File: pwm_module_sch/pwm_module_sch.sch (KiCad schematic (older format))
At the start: 47 parts, among them J1 SWIMM, J2 output -, J3 input, J4 output+, Q1 AO3400, Q2 6N60, SW1 ., SW2 ., U1 TM1637, U2 STM8S003F3P, U3 LM358, U4 L78L33

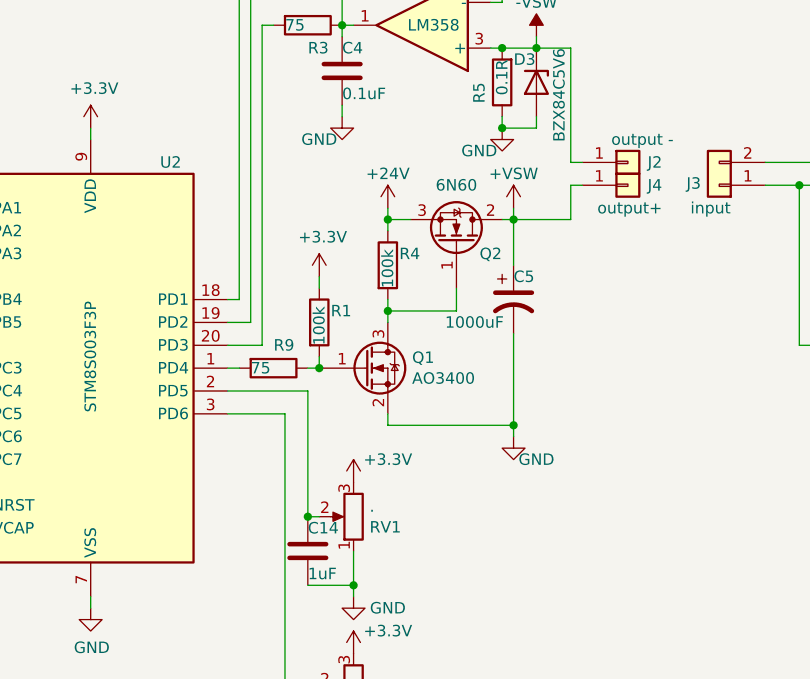
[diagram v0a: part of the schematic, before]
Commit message: low lewel written, not tested, todo: main menu
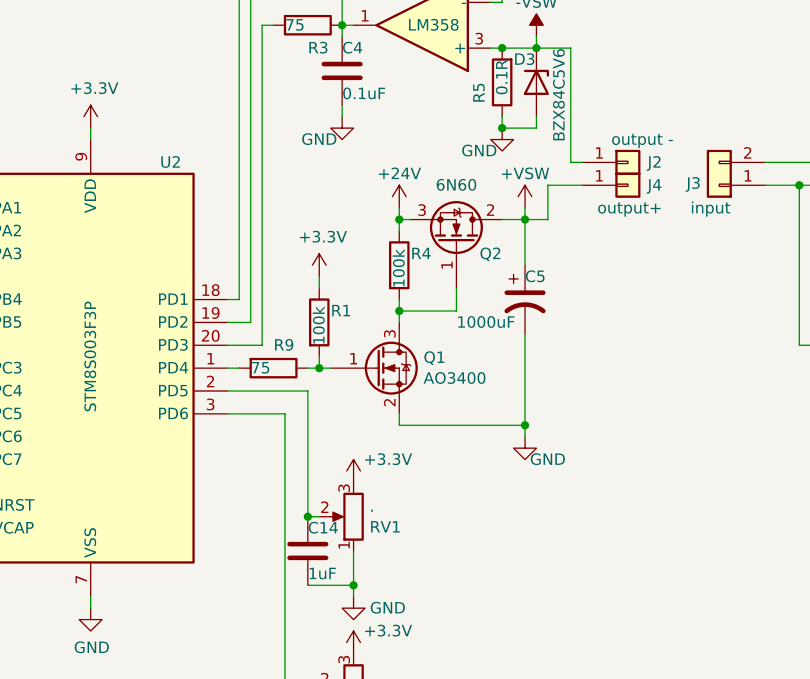
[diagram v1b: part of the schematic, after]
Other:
- moved on the sheet: C5, Q1, R4
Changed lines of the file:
@@
 L Device:R R4
 U 1 1 620AEA05
-P 4650 2800
-F 0 "R4" H 4700 2850 50  0000 L CNN
-F 1 "100k" V 4650 2700 50  0000 L CNN
-F 2 "Resistor_SMD:R_0402_1005Metric" V 4580 2800 50  0001 C CNN
-F 3 "~" H 4650 2800 50  0001 C CNN
-	1    4650 2800
-	1    0    0    -1
-$EndComp
-Wire Wire Line
-	4650 3050 4650 3000
-Connection ~ 4650 3000
-Wire Wire Line
-	4650 3000 4650 2950
+P 4700 2800
+F 0 "R4" H 4750 2850 50  0000 L CNN
+F 1 "100k" V 4700 2700 50  0000 L CNN
+F 2 "Resistor_SMD:R_0402_1005Metric" V 4630 2800 50  0001 C CNN
+F 3 "~" H 4700 2800 50  0001 C CNN
+	1    4700 2800
+	1    0    0    -1
+$EndComp
 $Comp
 L power:GND #PWR0105
@@
 	1    0    0    -1
 $EndComp
-Wire Wire Line
-	4650 3000 4950 3000
 $Comp
 L Device:R_Potentiometer RV1
@@
 	1    0    0    -1
 $EndComp
-Wire Wire Line
-	4350 2900 4350 2850
-Wire Wire Line
-	4650 2600 4650 2650
 $Comp
 L Amplifier_Operational:LM358 U3
@@
 L power:+VSW #PWR0112
 U 1 1 6218088D
-P 5200 2550
-F 0 "#PWR0112" H 5200 2400 50  0001 C CNN
-F 1 "+VSW" H 5200 2700 50  0000 C CNN
-F 2 "" H 5200 2550 50  0001 C CNN
-F 3 "" H 5200 2550 50  0001 C CNN
-	1    5200 2550
+P 5250 2550
+F 0 "#PWR0112" H 5250 2400 50  0001 C CNN
+F 1 "+VSW" H 5250 2700 50  0000 C CNN
+F 2 "" H 5250 2550 50  0001 C CNN
+F 3 "" H 5250 2550 50  0001 C CNN
+	1    5250 2550
 	1    0    0    -1
 $EndComp
@@
 L power:+24V #PWR0113
 U 1 1 6218BBB0
-P 4650 2550
-F 0 "#PWR0113" H 4650 2400 50  0001 C CNN
-F 1 "+24V" H 4650 2700 50  0000 C CNN
-F 2 "" H 4650 2550 50  0001 C CNN
-F 3 "" H 4650 2550 50  0001 C CNN
-	1    4650 2550
-	1    0    0    -1
-$EndComp
-Wire Wire Line
-	4650 2600 4650 2550
-Connection ~ 4650 2600
-Wire Wire Line
-	4750 2600 4650 2600
-Wire Wire Line
-	4950 2900 4950 3000
-Wire Wire Line
-	5150 2600 5200 2600
-Wire Wire Line
-	5200 2600 5200 2550
+P 4700 2550
+F 0 "#PWR0113" H 4700 2400 50  0001 C CNN
+F 1 "+24V" H 4700 2700 50  0000 C CNN
+F 2 "" H 4700 2550 50  0001 C CNN
+F 3 "" H 4700 2550 50  0001 C CNN
+	1    4700 2550
+	1    0    0    -1
+$EndComp
 $Comp
 L power:+3.3V #PWR0114
@@
 	1    0    0    -1
 $EndComp
-Connection ~ 5200 2600
 $Comp
 L Device:C_Polarized_US C5
 U 1 1 62166329
-P 5200 2950
-F 0 "C5" H 5200 3050 50  0000 L CNN
-F 1 "1000uF" H 4900 2850 50  0000 L CNN
-F 2 "Capacitor_THT:CP_Radial_D5.0mm_P2.00mm" H 5200 2950 50  0001 C CNN
-F 3 "~" H 5200 2950 50  0001 C CNN
-	1    5200 2950
-	1    0    0    -1
-$EndComp
-Wire Wire Line
-	5200 2800 5200 2600
+P 5250 2950
+F 0 "C5" H 5250 3050 50  0000 L CNN
+F 1 "1000uF" H 4950 2850 50  0000 L CNN
+F 2 "Capacitor_THT:CP_Radial_D5.0mm_P2.00mm" H 5250 2950 50  0001 C CNN
+F 3 "~" H 5250 2950 50  0001 C CNN
+	1    5250 2950
+	1    0    0    -1
+$EndComp
 $Comp
 L Device:R R2
@@
 Wire Wire Line
 	5300 1850 5450 1850
-Wire Wire Line
-	5450 1850 5450 2350
-Wire Wire Line
-	5450 2350 5500 2350
 Connection ~ 5300 1850
-Wire Wire Line
-	5450 2600 5450 2450
-Wire Wire Line
-	5200 2600 5450 2600
-Wire Wire Line
-	5450 2450 5500 2450
 Wire Wire Line
 	4050 1050 4100 1050
@@
 	0    1    1    0
 $EndComp
-Wire Wire Line
-	4350 3250 4350 3200
 $Comp
 L Connector_Generic:Conn_01x01 J4
@@
 L power:GND #PWR0129
 U 1 1 62235D6C
-P 5200 3550
-F 0 "#PWR0129" H 5200 3300 50  0001 C CNN
-F 1 "GND" H 5300 3450 50  0000 C CNN
-F 2 "" H 5200 3550 50  0001 C CNN
-F 3 "" H 5200 3550 50  0001 C CNN
-	1    5200 3550
+P 5250 3550
+F 0 "#PWR0129" H 5250 3300 50  0001 C CNN
+F 1 "GND" H 5350 3450 50  0000 C CNN
+F 2 "" H 5250 3550 50  0001 C CNN
+F 3 "" H 5250 3550 50  0001 C CNN
+	1    5250 3550
 	1    0    0    -1
 $EndComp
@@
 	2200 3050 2200 6250
 Wire Wire Line
-	5200 3500 5200 3100
-Wire Wire Line
 	4200 3450 4200 4650
 Wire Wire Line
-	4350 3250 4300 3250
-Wire Wire Line
 	4000 3250 3950 3250
-Wire Wire Line
-	3950 3350 4300 3350
-Wire Wire Line
-	4300 3350 4300 3900
-Connection ~ 4300 3900
-Connection ~ 4350 3250
 $Comp
 L local:AO3400 Q1
 U 1 1 620ABAF0
-P 4550 3250
-F 0 "Q1" H 4756 3296 50  0000 L CNN
-F 1 "AO3400" H 4756 3205 50  0000 L CNN
-F 2 "Package_TO_SOT_SMD:SOT-23" H 4550 3250 50  0001 C CNN
-F 3 "" H 4550 3250 50  0001 L CNN
-	1    4550 3250
-	1    0    0    -1
-$EndComp
-Wire Wire Line
-	4650 3450 4650 3500
-Wire Wire Line
-	4650 3500 5200 3500
-Wire Wire Line
-	5200 3550 5200 3500
-Connection ~ 5200 3500
+P 4600 3250
+F 0 "Q1" H 4806 3296 50  0000 L CNN
+F 1 "AO3400" H 4806 3205 50  0000 L CNN
+F 2 "Package_TO_SOT_SMD:SOT-23" H 4600 3250 50  0001 C CNN
+F 3 "" H 4600 3250 50  0001 L CNN
+	1    4600 3250
+	1    0    0    -1
+$EndComp
 $Comp
 L Device:R R11
@@
 Wire Wire Line
 	2300 5900 2300 5850
+Wire Wire Line
+	4350 3200 4350 3250
+Wire Wire Line
+	4350 3250 4400 3250
+Wire Wire Line
+	4300 3250 4350 3250
+Connection ~ 4350 3250
+Wire Wire Line
+	4350 2900 4350 2850
+Wire Wire Line
+	4700 3450 4700 3500
+Wire Wire Line
+	4950 2900 4950 3000
+Wire Wire Line
+	4950 3000 4700 3000
+Wire Wire Line
+	4700 3000 4700 3050
+Wire Wire Line
+	4700 2950 4700 3000
+Connection ~ 4700 3000
+Wire Wire Line
+	4700 2650 4700 2600
+Wire Wire Line
+	4750 2600 4700 2600
+Connection ~ 4700 2600
+Wire Wire Line
+	4700 2600 4700 2550
+Wire Wire Line
+	5150 2600 5250 2600
+Wire Wire Line
+	5250 3500 5250 3550
+Wire Wire Line
+	4700 3500 5250 3500
+Wire Wire Line
+	5250 3100 5250 3500
+Connection ~ 5250 3500
+Wire Wire Line
+	5250 2800 5250 2600
+Connection ~ 5250 2600
+Wire Wire Line
+	5250 2600 5250 2550
+Wire Wire Line
+	5450 1850 5450 2350
+Wire Wire Line
+	5450 2350 5500 2350
+Wire Wire Line
+	5250 2600 5350 2600
+Wire Wire Line
+	5350 2600 5350 2450
+Wire Wire Line
+	5350 2450 5500 2450
+Wire Wire Line
+	4300 3900 4300 3350
+Wire Wire Line
+	4300 3350 3950 3350
+Connection ~ 4300 3900
 $EndSCHEMATC
